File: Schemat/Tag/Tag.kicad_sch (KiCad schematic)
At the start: 12 parts, among them U1 SX1276, U2 ESP32-S3, Y1 ABM8G-32.000MHZ-B4Y-T

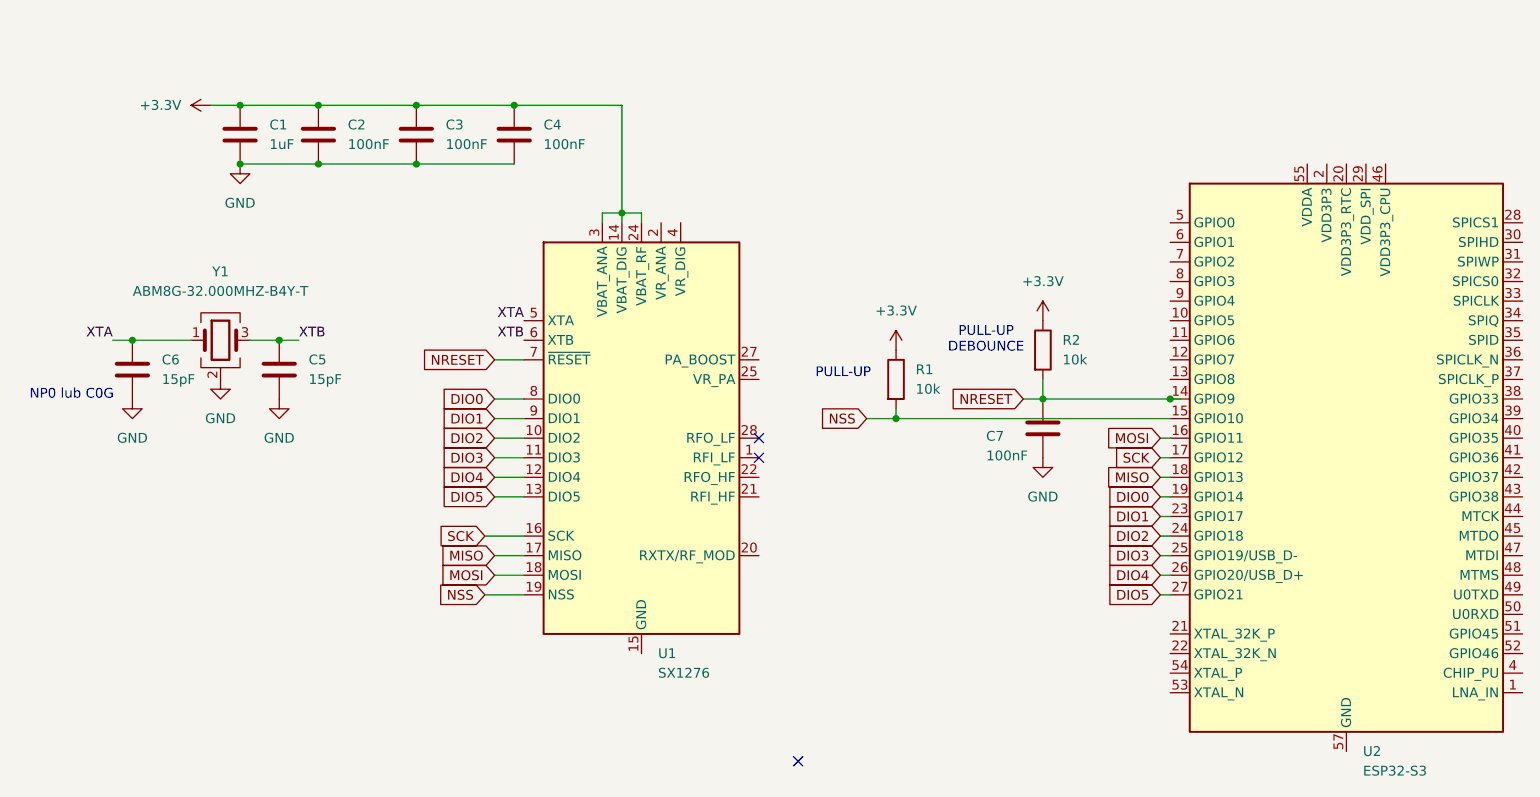
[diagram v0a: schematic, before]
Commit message: Wesja Beta skończona do weryfikacji
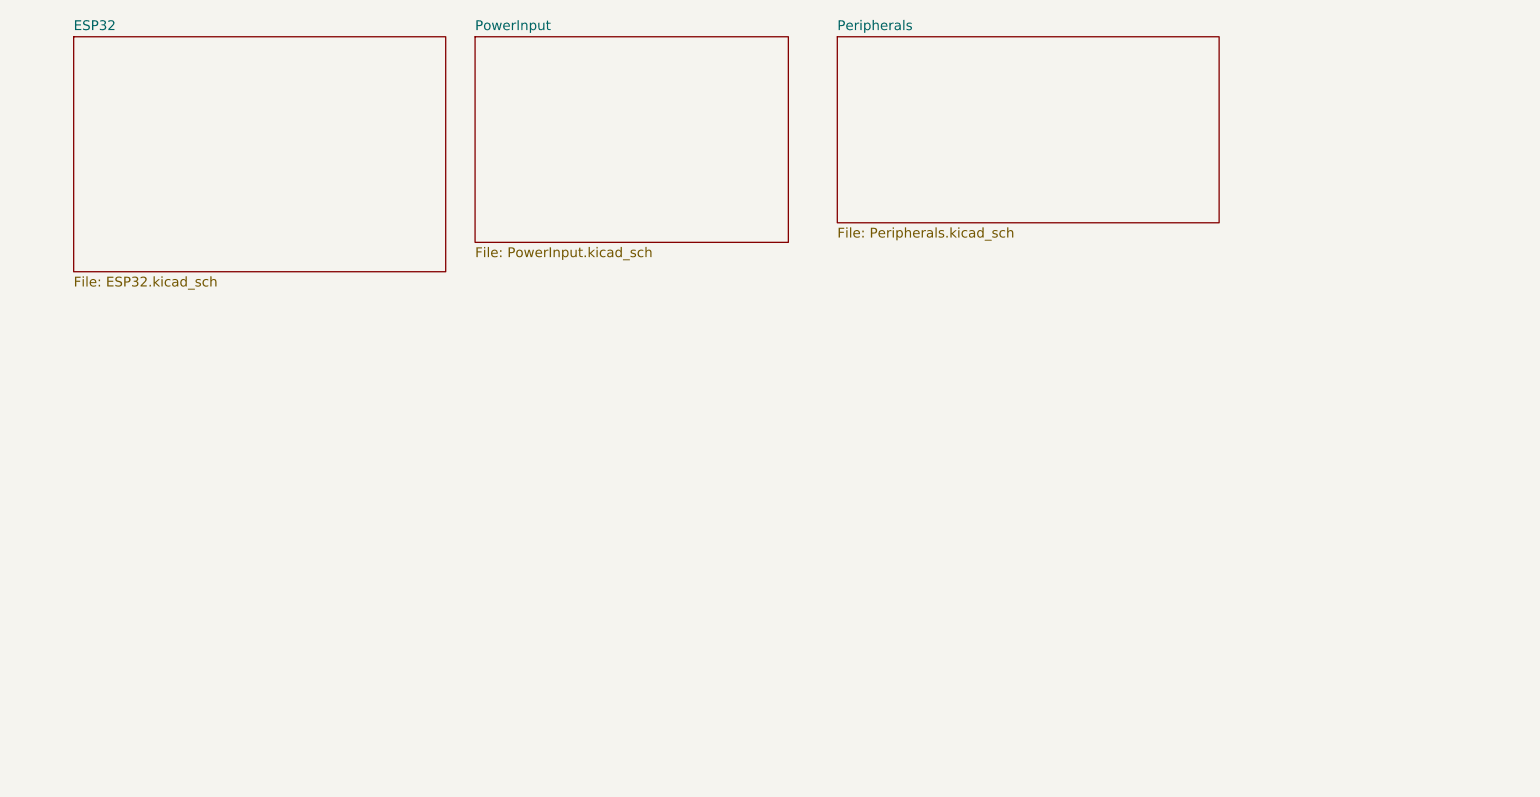
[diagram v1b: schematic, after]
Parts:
- removed C1: 1uF, symbol Device:C
- removed C2, C3, C4, C7: 100nF, symbol Device:C
- removed C5, C6: 15pF, symbol Device:C
- removed R1, R2: 10k, symbol Device:R
- removed U1: SX1276, Package_DFN_QFN:QFN-28-1EP_6x6mm_P0.65mm_EP4.8x4.8mm, symbol RF:SX1276
- removed U2: ESP32-S3, Package_DFN_QFN:QFN-56-1EP_7x7mm_P0.4mm_EP4x4mm, symbol MCU_Espressif:ESP32-S3
- removed Y1: ABM8G-32.000MHZ-B4Y-T, symbol Device:Crystal_GND24
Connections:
- no-connect marks 3 -> 0
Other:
- added sheet ESP32 (ESP32.kicad_sch)
- added sheet Peripherals (Peripherals.kicad_sch)
- added sheet PowerInput (PowerInput.kicad_sch)
- note removed: "NP0 lub C0G"
- note removed: "PULL-UP"
- note removed: "PULL-UP DEBOUNCE"
